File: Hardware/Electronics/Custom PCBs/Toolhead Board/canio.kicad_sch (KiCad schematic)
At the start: 11 parts, among them J1 120TR, J3 CAN, U6 SN65HVD1050D

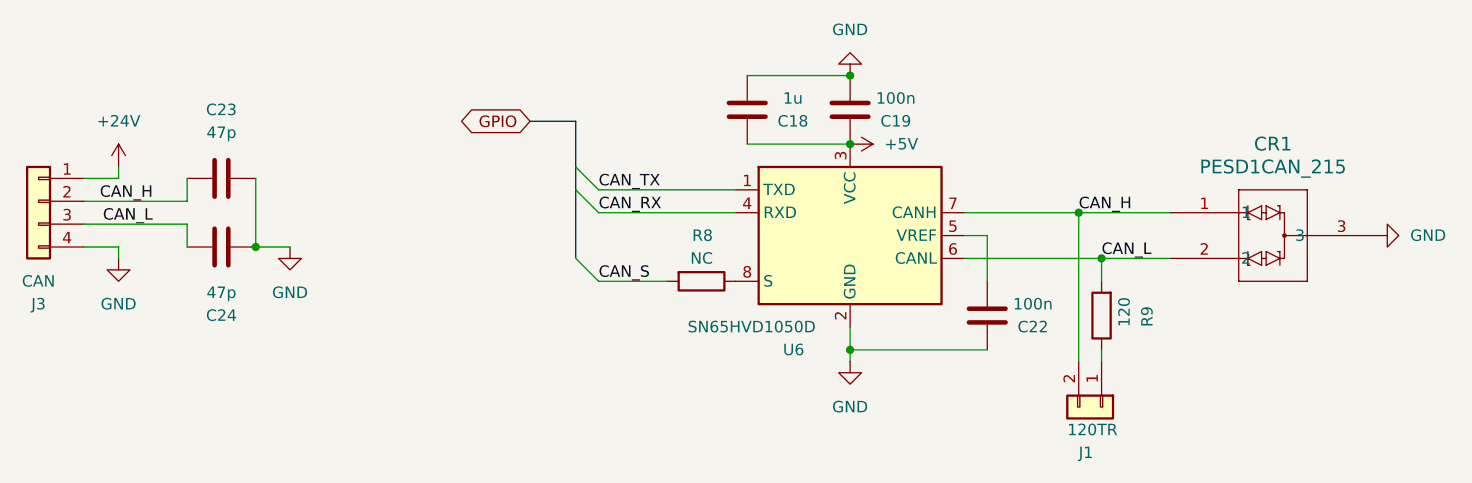
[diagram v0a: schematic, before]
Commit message: some updates
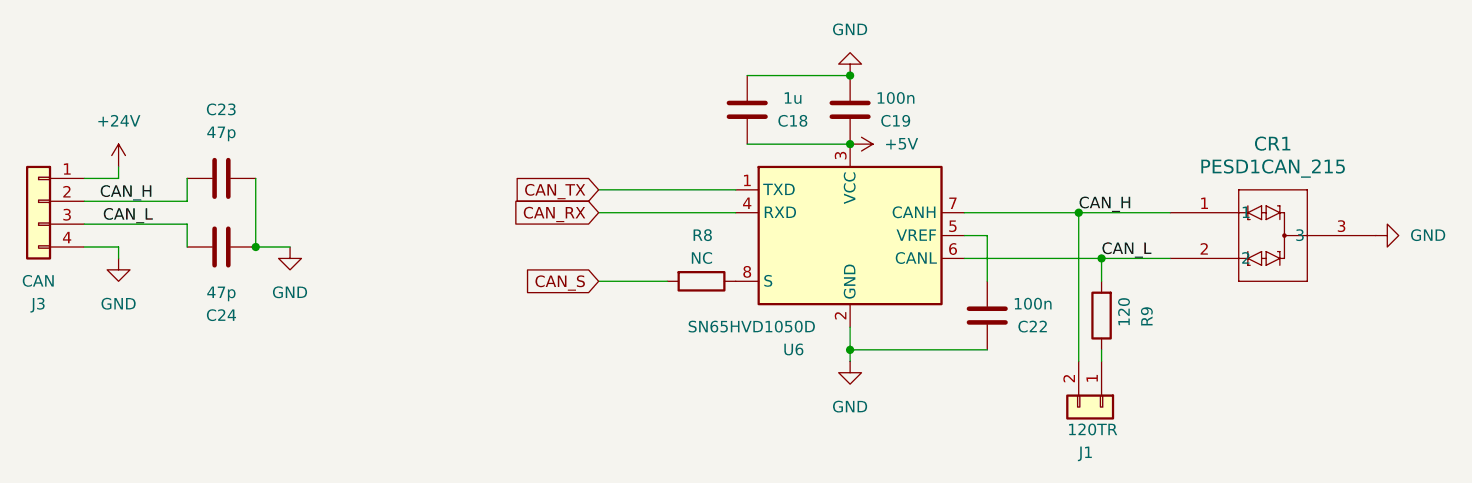
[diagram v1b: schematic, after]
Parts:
- C18, C19, C22: footprint Capacitor_SMD:C_0402_1005Metric -> (none)
- C23, C24: footprint Capacitor_SMD:C_0402_1005Metric -> (none); LCSC C881999 -> (none)
- CR1: footprint Package_TO_SOT_SMD:SOT-23 -> (none)
- J1: footprint Connector_PinHeader_2.54mm:PinHeader_1x02_P2.54mm_Vertical -> (none)
- J3: footprint Connector_JST:JST_PH_S4B-PH-K_1x04_P2.00mm_Horizontal -> (none)
- R8, R9: footprint Resistor_SMD:R_0402_1005Metric -> (none); LCSC C966873 -> (none)
- U6: footprint Package_SO:SOIC-8_3.9x4.9mm_P1.27mm -> (none)
